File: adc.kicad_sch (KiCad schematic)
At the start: 27 parts, among them U7 AD7177-2BRUZ, U70 TG2520SMN-16M-MCG, U75 OPA2189DGK

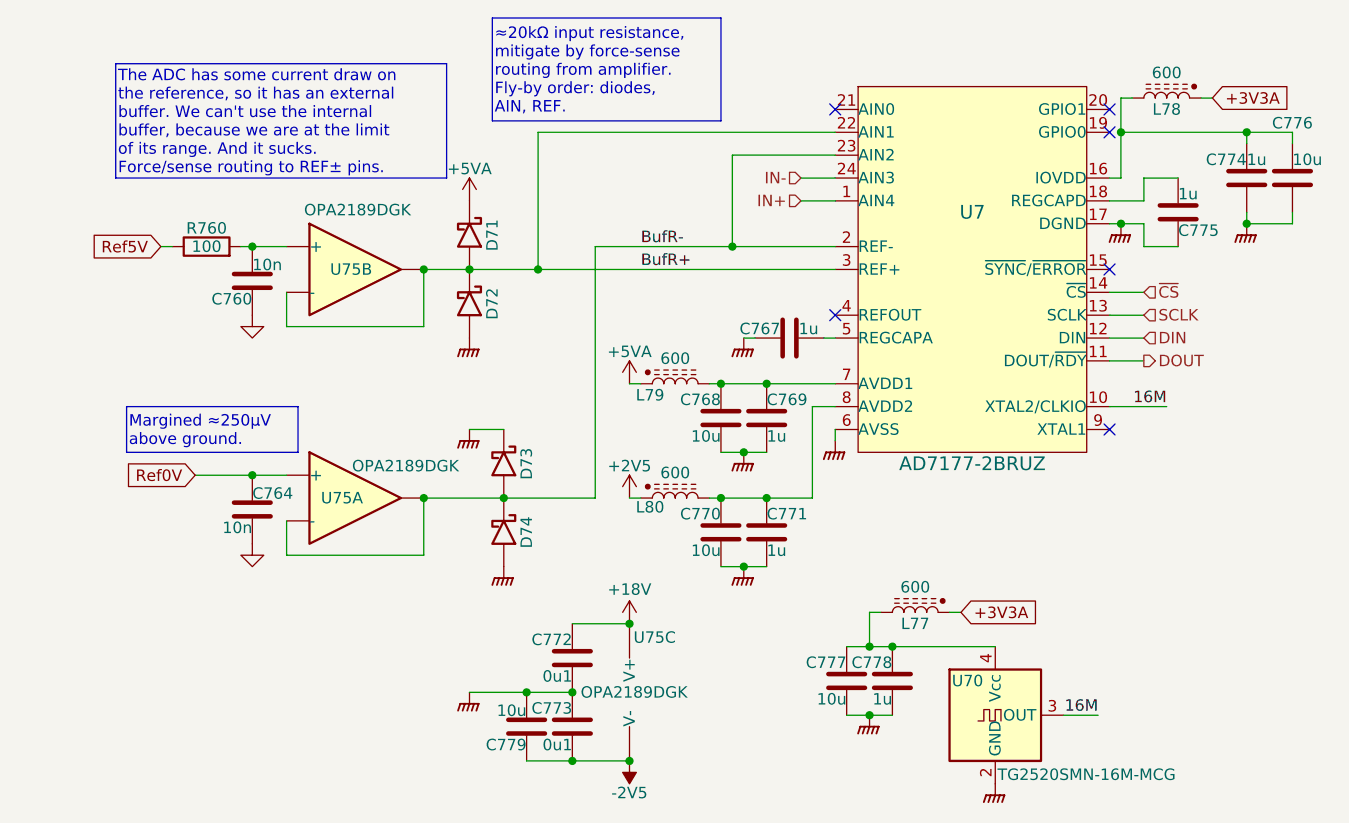
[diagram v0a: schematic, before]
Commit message: About to delete scan...
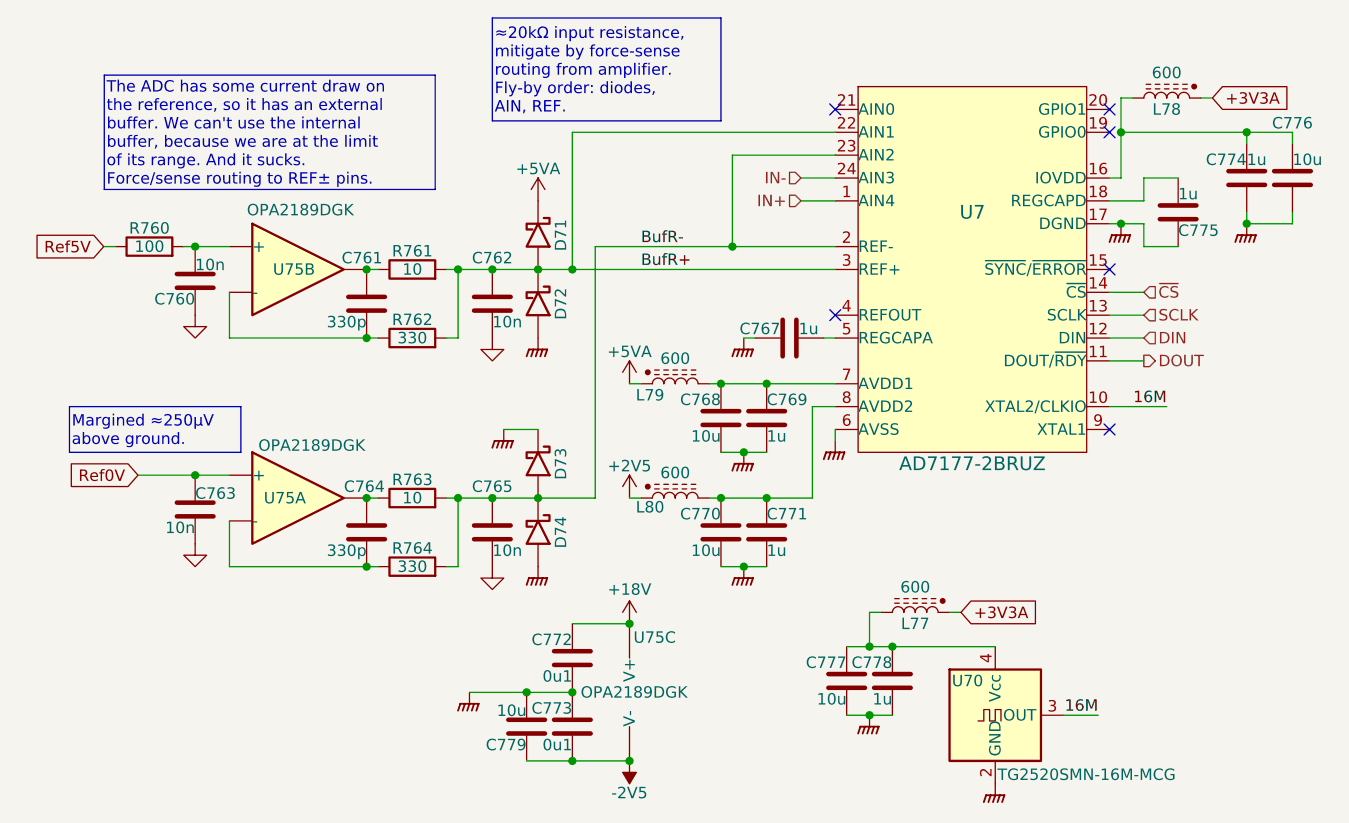
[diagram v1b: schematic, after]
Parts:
- added C761, C764: 330p, Capacitor_SMD:C_0603_1608Metric, symbol Device:C
- added C762, C765: 10n, Capacitor_SMD:C_0603_1608Metric, symbol Device:C
- added R761, R763: 10, Resistor_SMD:R_0402_1005Metric, symbol Device:R
- added R762, R764: 330, Resistor_SMD:R_0402_1005Metric, symbol Device:R
- R760: LCSC (none) -> C25076
- U7: Stock (none) -> 1
- U70: footprint Oscillator:Oscillator_SMD_SeikoEpson_TG2520SMN-xxx-xxxxxx-4Pin_2.5x2.0mm -> Parts:TG2520SMN
- U75: Stock (none) -> 15
- renumbered C764 to C763
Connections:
- net BufR+: now also C762.1, R761.2, R762.2; no longer U75.6 (-), U75.7
- net BufR-: now also C765.1, R763.2, R764.2; no longer U75.1, U75.2 (-)
- net GND: now also C762.2, C765.2
- new net: C764.1, R763.1, U75.1
- new net: C764.2, R764.1, U75.2 (-)
- new net: C761.2, R762.1, U75.6 (-)
- new net: C761.1, R761.1, U75.7
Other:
- moved on the sheet: C760, C763, D71, D72, D73, D74, R760, U75A, U75B
